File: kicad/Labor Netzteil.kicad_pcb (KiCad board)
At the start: 2 copper layers, 95.2 x 97.8 mm, 44 parts, among them J1 Out_1_01, J10 Sec 2 d, J11 Out_2_02, J12 Out_2_01, J13 OLED, J14 Fan, J15 Out_1, J16 NeoPixel, J17 Out_2, J2 Out_1_02, J3 Sec 1 d, J4 Sec 1 c, J5 Sec 1 b, J6 Sec 1 a, J7 Sec 2 a, J8 Sec 2 b, J9 Sec 2 c, U1 2-Relais-Modul, U2 LM7805_TO220, U3 L7812, U4 ESP-DevKitC, U5 74HC245, U6 DS18B20

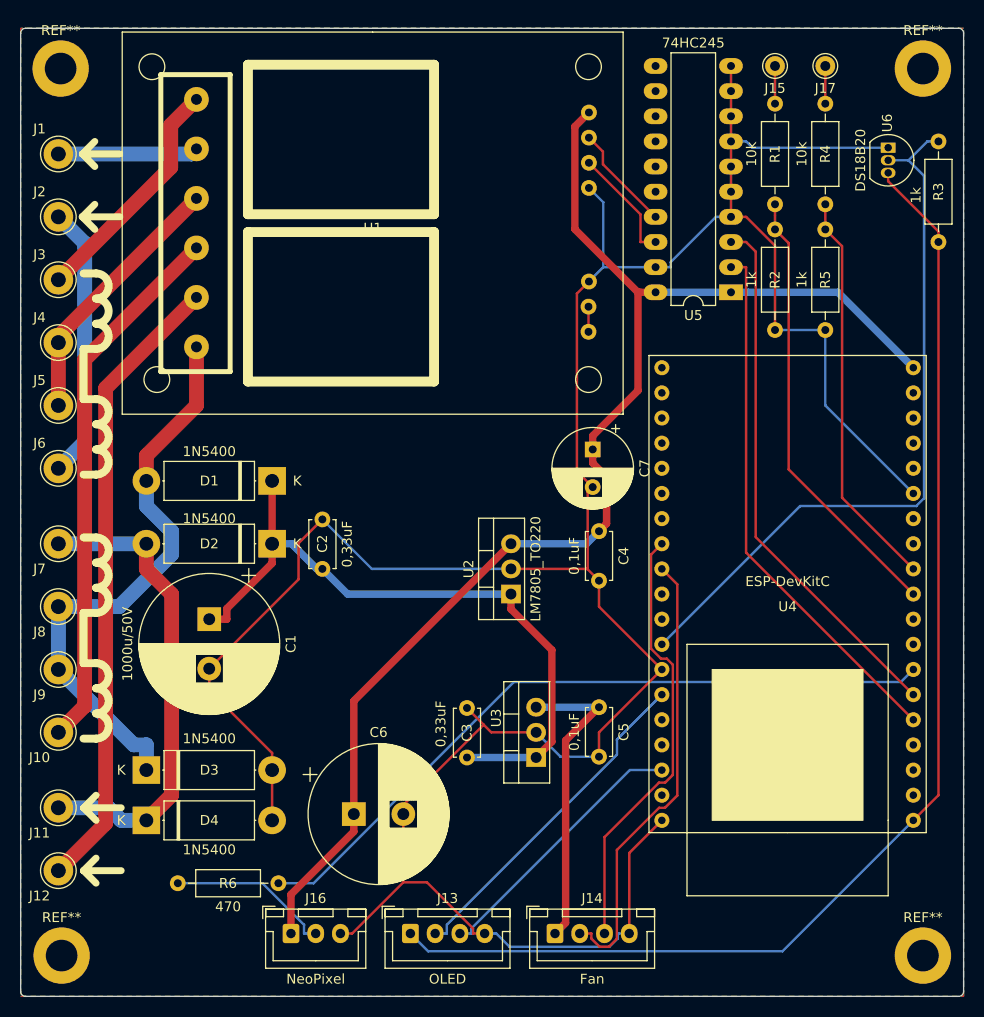
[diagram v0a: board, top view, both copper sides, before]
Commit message: Neueste Änderungen
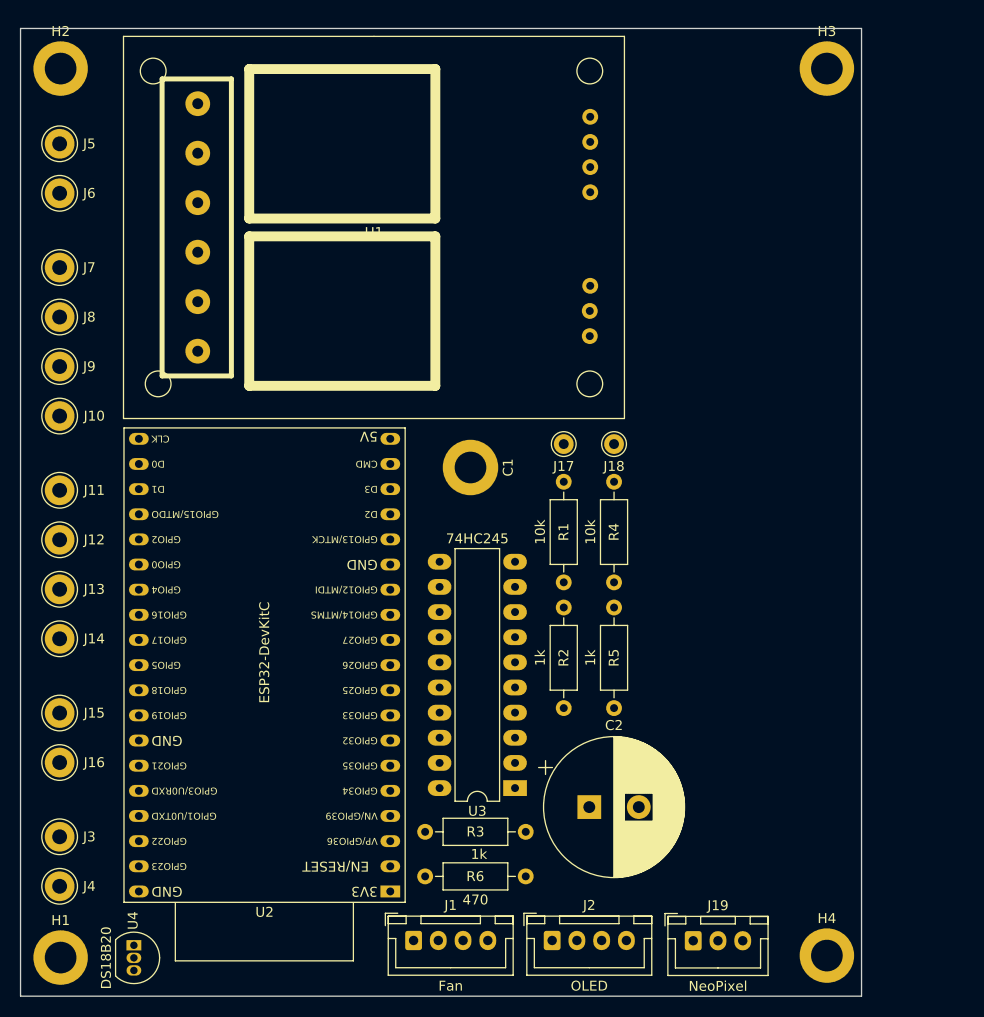
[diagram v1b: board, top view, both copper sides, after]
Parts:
- removed the C1 at (118.1, 96.5)
- removed C3: 0,33uF, Capacitor_THT:C_Disc_D4.7mm_W2.5mm_P5.00mm
- removed C4, C5: 0,1uF, Capacitor_THT:C_Disc_D4.7mm_W2.5mm_P5.00mm
- removed C6: 1000uF, Capacitor_THT:CP_Radial_D14.0mm_P5.00mm
- removed D1, D2, D3, D4: 1N5400, Diode_THT:D_5W_P12.70mm_Horizontal
- removed REF** (x4): MountingHole_3.2mm_M3_ISO7380_Pad, MountingHole:MountingHole_3.2mm_M3_ISO7380_Pad
- removed the U3 at (151.1, 110.5)
- removed the U4 at (176.5, 94.0)
- added H1: MountingHole_Pad, MountingHole:MountingHole_3.2mm_M3_ISO14580_Pad, F.Cu at (103.1, 130.7)
- added H2: MountingHole_Pad, MountingHole:MountingHole_3.2mm_M3_ISO14580_Pad, F.Cu at (103.1, 40.9)
- added H3: MountingHole_Pad, MountingHole:MountingHole_3.2mm_M3_ISO14580_Pad, F.Cu at (180.5, 40.9)
- added H4: MountingHole_Pad, MountingHole:MountingHole_3.2mm_M3_ISO14580_Pad, F.Cu at (180.5, 130.5)
- added J3: +5V In, Connector_Pin:Pin_D1.3mm_L11.0mm_LooseFit, F.Cu at (103.0, 118.5)
- added J4: GND 5V In, Connector_Pin:Pin_D1.3mm_L11.0mm_LooseFit, F.Cu at (103.0, 123.5)
- C1: renamed from C7; footprint Capacitor_THT:CP_Radial_D8.0mm_P3.80mm -> MountingHole:MountingHole_3.2mm_M3_DIN965_Pad
- C2: value 0,33uF -> 1000uF; footprint Capacitor_THT:C_Disc_D4.7mm_W2.5mm_P5.00mm -> Capacitor_THT:CP_Radial_D14.0mm_P5.00mm
- U2: value LM7805_TO220 -> ESP32-DevKitC; footprint Package_TO_SOT_THT:TO-220-3_Vertical -> PCM_Espressif:ESP32-DevKitC
- moved U4 110.9 mm to (110.5, 129.5)
- moved R3 72.7 mm to (150.1, 118.0), turned to 180 degrees
- moved U3 54.6 mm to (149.0, 113.6)
- moved R2 43.7 mm to (153.9, 95.3)
- moved R5 43.7 mm to (159.0, 95.3)
- moved J17 43.7 mm to (153.9, 78.8)
- moved J18 43.7 mm to (159.0, 78.8)
- moved R1 43.7 mm to (153.9, 82.6)
- moved R4 43.7 mm to (159.0, 82.6)
- moved J19 40.6 mm to (167.0, 129.0)
- moved C2 36.1 mm to (156.5, 115.5), turned to 0 degrees
- moved U2 32.4 mm to (136.4, 124.0), turned to 180 degrees
- moved R6 25.0 mm to (139.9, 122.5)
- moved J2 14.3 mm to (152.8, 129.0)
- moved J1 14.3 mm to (138.8, 129.0)
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- renumbered J14 to J1, J6 to J10, J7 to J11, J8 to J12, J9 to J13, J10 to J14, J11 to J15, J12 to J16, J15 to J17, J17 to J18, J16 to J19, J13 to J2, J1 to J5, J2 to J6, J3 to J7, J4 to J8, J5 to J9, U5 to U3, U6 to U4
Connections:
- C2 pad 1: Net-(C1-Pad1) -> 5V
- J1 pad 1: 12V -> 5V
- J2 pad 1: 3V3 -> 5V
- R3 pad 1: 3V3 -> 5V
- U1 pad 7: Net-(U1-Pad7) -> 5V
- U1 pad 8: Net-(U1-Pad7) -> 5V
- U2 pad 1: Net-(C1-Pad1) -> unconnected-(U2-3V3-Pad1)
- U2 pad 2: GND -> unconnected-(U2-CHIP_PU-Pad2)
- U2 pad 3: 5V -> unconnected-(U2-SENSOR_VP/GPIO36/ADC1_CH0-Pad3)
- U3 pad 11: Net-(U5-Pad11) -> unconnected-(U3-B7-Pad11)
- U3 pad 12: Net-(U5-Pad12) -> unconnected-(U3-B6-Pad12)
- U3 pad 13: Net-(U5-Pad13) -> unconnected-(U3-B5-Pad13)
- U3 pad 14: Net-(U5-Pad14) -> unconnected-(U3-B4-Pad14)
- U3 pad 15: Net-(U5-Pad15) -> unconnected-(U3-B3-Pad15)
- U3 pad 16: Net-(U5-Pad16) -> NeoPixel
- U3 pad 4: GND -> A2
- U4 pad 3: 3V3 -> 5V
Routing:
- net GND: track 301.1 -> 0.00 mm
- net 5V: track 137.3 -> 0.00 mm
- net 3V3: track 125.6 -> 0.00 mm
- net DS18B20: track 73.3 -> 0.00 mm
- net NeoPixel: track 73.1 -> 0.00 mm
- net Net-(C1-Pad1): track 69.7 -> 0.00 mm
- net Net-(J16-Pin_1): track 63.7 -> 0.00 mm
- net Net-(J12-Pin_1): track 58.7 -> 0.00 mm
- net Net-(J14-Pin_1): track 54.7 -> 0.00 mm
- net A1: track 54.2 -> 0.00 mm
- net A0: track 54.2 -> 0.00 mm
- net Net-(J11-Pin_1): track 48.4 -> 0.00 mm
- net TACHO: track 45.8 -> 0.00 mm
- net V_MON_1: track 45.2 -> 0.00 mm
- net PWM: track 44.3 -> 0.00 mm
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- removed copper zone on B.Cu, net GND
- removed copper zone on F.Cu, net GND
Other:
- board size 95.2 x 97.8 mm -> 85 x 97.8 mm

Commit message: Grundlegende Änderung der Schaltung, siehe README
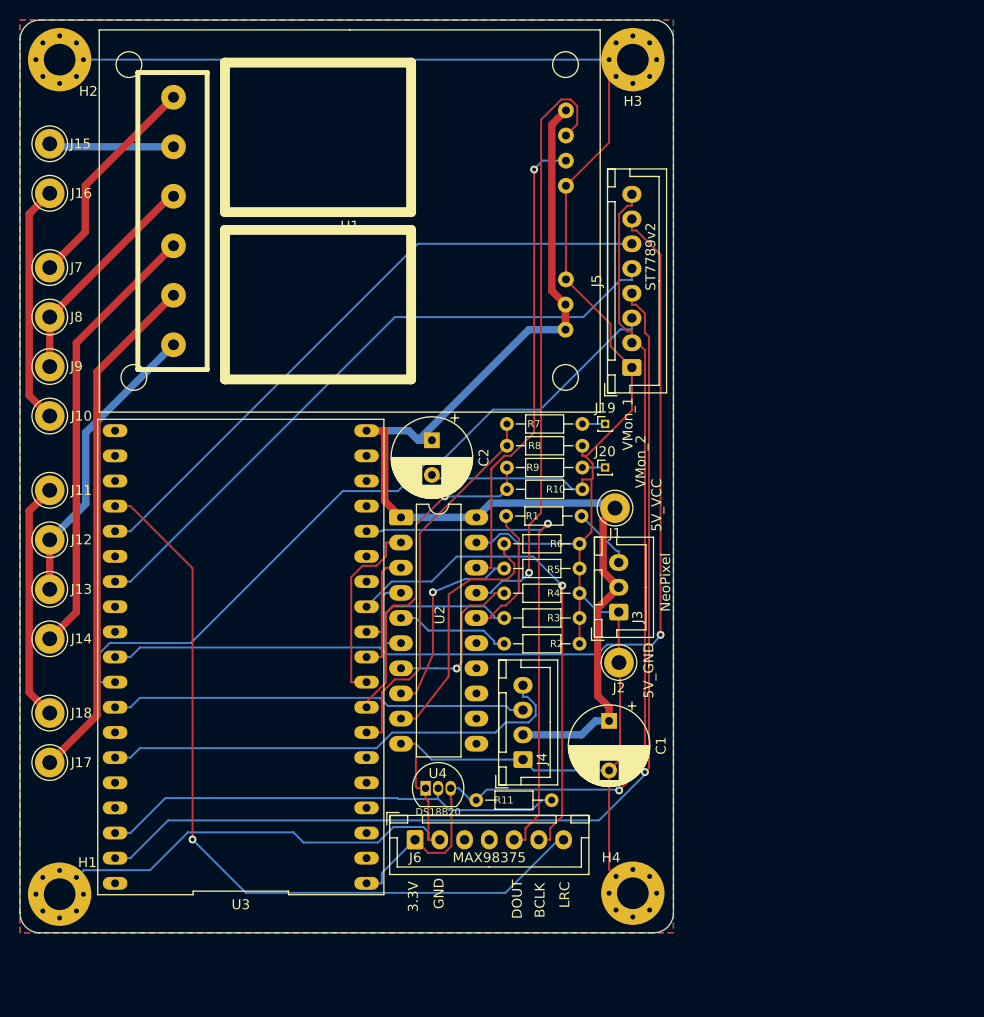
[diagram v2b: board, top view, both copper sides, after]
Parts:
- removed the J3 at (103.0, 118.5)
- added J5: ST7789v2, Connector_JST:JST_XH_B8B-XH-A_1x08_P2.50mm_Vertical, F.Cu at (160.8, 71.1)
- added J6: MAX98375, Connector_JST:JST_XH_B7B-XH-A_1x07_P2.50mm_Vertical, F.Cu at (138.9, 118.8)
- added R2: 10K, Resistor_THT:R_Axial_DIN0204_L3.6mm_D1.6mm_P7.62mm_Horizontal, F.Cu at (155.5, 99.0)
- added R3: 10K, Resistor_THT:R_Axial_DIN0204_L3.6mm_D1.6mm_P7.62mm_Horizontal, F.Cu at (155.5, 96.4)
- added R4: 10K, Resistor_THT:R_Axial_DIN0204_L3.6mm_D1.6mm_P7.62mm_Horizontal, F.Cu at (155.5, 93.9)
- added R5: 10K, Resistor_THT:R_Axial_DIN0204_L3.6mm_D1.6mm_P7.62mm_Horizontal, F.Cu at (155.5, 91.4)
- added R6: 10K, Resistor_THT:R_Axial_DIN0204_L3.6mm_D1.6mm_P7.62mm_Horizontal, F.Cu at (155.5, 88.9)
- C1: renamed from C2; footprint Capacitor_THT:CP_Radial_D14.0mm_P5.00mm -> Capacitor_THT:CP_Radial_D8.0mm_P5.00mm
- C2: renamed from C1; footprint MountingHole:MountingHole_3.2mm_M3_DIN965_Pad -> Capacitor_THT:CP_Radial_D8.0mm_P3.50mm
- H1: value MountingHole_Pad -> H1; footprint MountingHole:MountingHole_3.2mm_M3_ISO14580_Pad -> MountingHole:MountingHole_3.2mm_M3_Pad_Via
- H2: value MountingHole_Pad -> H2; footprint MountingHole:MountingHole_3.2mm_M3_ISO14580_Pad -> MountingHole:MountingHole_3.2mm_M3_Pad_Via
- H3: value MountingHole_Pad -> H3; footprint MountingHole:MountingHole_3.2mm_M3_ISO14580_Pad -> MountingHole:MountingHole_3.2mm_M3_Pad_Via
- H4: value MountingHole_Pad -> H4; footprint MountingHole:MountingHole_3.2mm_M3_ISO14580_Pad -> MountingHole:MountingHole_3.2mm_M3_Pad_Via
- J1: value Fan -> 5V_VCC; footprint Connector_JST:JST_XH_B4B-XH-A_1x04_P2.50mm_Vertical -> Connector_Pin:Pin_D1.3mm_L11.0mm_LooseFit
- J19: renamed from J17; value Out_1 -> VMon_1; footprint Connector_Pin:Pin_D1.0mm_L10.0mm -> Connector_PinHeader_1.00mm:PinHeader_1x01_P1.00mm_Vertical
- J2: value OLED -> 5V_GND; footprint Connector_JST:JST_XH_B4B-XH-A_1x04_P2.50mm_Vertical -> Connector_Pin:Pin_D1.3mm_L11.0mm_LooseFit
- J20: renamed from J18; value Out_2 -> VMon_2; footprint Connector_Pin:Pin_D1.0mm_L10.0mm -> Connector_PinHeader_1.00mm:PinHeader_1x01_P1.00mm_Vertical
- J4: value GND 5V In -> Fan; footprint Connector_Pin:Pin_D1.3mm_L11.0mm_LooseFit -> Connector_JST:JST_XH_B4B-XH-A_1x04_P2.50mm_Vertical
- R1: renamed from R6; footprint Resistor_THT:R_Axial_DIN0207_L6.3mm_D2.5mm_P10.16mm_Horizontal -> Resistor_THT:R_Axial_DIN0204_L3.6mm_D1.6mm_P7.62mm_Horizontal
- R10: renamed from R5; footprint Resistor_THT:R_Axial_DIN0207_L6.3mm_D2.5mm_P10.16mm_Horizontal -> Resistor_THT:R_Axial_DIN0204_L3.6mm_D1.6mm_P7.62mm_Horizontal
- R11: renamed from R3; value 1k -> 4.7K; footprint Resistor_THT:R_Axial_DIN0207_L6.3mm_D2.5mm_P10.16mm_Horizontal -> Resistor_THT:R_Axial_DIN0204_L3.6mm_D1.6mm_P7.62mm_Horizontal
- R7: renamed from R1; footprint Resistor_THT:R_Axial_DIN0207_L6.3mm_D2.5mm_P10.16mm_Horizontal -> Resistor_THT:R_Axial_DIN0204_L3.6mm_D1.6mm_P7.62mm_Horizontal
- R8: renamed from R2; footprint Resistor_THT:R_Axial_DIN0207_L6.3mm_D2.5mm_P10.16mm_Horizontal -> Resistor_THT:R_Axial_DIN0204_L3.6mm_D1.6mm_P7.62mm_Horizontal
- R9: renamed from R4; footprint Resistor_THT:R_Axial_DIN0207_L6.3mm_D2.5mm_P10.16mm_Horizontal -> Resistor_THT:R_Axial_DIN0204_L3.6mm_D1.6mm_P7.62mm_Horizontal
- U2: value ESP32-DevKitC -> 74HC245; footprint PCM_Espressif:ESP32-DevKitC -> Package_DIP:DIP-20_W7.62mm_LongPads
- U3: value 74HC245 -> ESP32-DEVKITC-32D; footprint Package_DIP:DIP-20_W7.62mm_LongPads -> RF_Module:ESP32-DevKitC-V4-b
- moved J4 48.5 mm to (149.8, 110.7), turned to 90 degrees
- moved J1 48.2 mm to (159.1, 85.3)
- moved R1 39.7 mm to (155.7, 86.1), turned to 180 degrees
- moved U2 37.8 mm to (137.5, 86.2), turned to 0 degrees
- moved J3 34.0 mm to (159.5, 95.8), turned to 90 degrees
- moved U4 33.5 mm to (140.0, 113.6), turned to 0 degrees
- moved U3 30.7 mm to (121.3, 100.3), turned to 90 degrees
- moved J2 28.9 mm to (159.5, 100.9)
- moved H4 20.6 mm to (160.9, 124.2)
- moved H3 19.6 mm to (160.9, 40.0)
- moved R8 17.3 mm to (148.2, 79.0), turned to 0 degrees
- moved R10 16.1 mm to (148.2, 83.4), turned to 0 degrees
- moved C1 8.93 mm to (158.5, 106.8), turned to -90 degrees
- moved H1 6.40 mm to (103.0, 124.3)
- moved R7 6.14 mm to (155.8, 76.8), turned to 180 degrees
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- renumbered J5 to J15, J6 to J16, J16 to J17, J15 to J18, J19 to J3
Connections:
- J2 pad 1: 5V -> GND
- J3 pad 1: 5V -> GND
- J3 pad 2: Net-(J19-Pin_2) -> 5V
- J3 pad 3: GND -> Net-(J3-Pin_3)
- R1 pad 1: Net-(J19-Pin_2) -> Net-(J3-Pin_3)
- R1 pad 2: NeoPixel -> NP_5V
- R11 pad 1: 5V -> 3.3V
- U2 pad 1: unconnected-(U2-3V3-Pad1) -> 5V
- U2 pad 10: V_MON_1 -> GND
- U2 pad 11: V_MON_2 -> unconnected-(U2-B7-Pad11)
- U2 pad 14: GND -> unconnected-(U2-B4-Pad14)
- U2 pad 16: unconnected-(U2-SD_DATA2/GPIO9-Pad16) -> NP_5V
- U2 pad 17: unconnected-(U2-SD_DATA3/GPIO10-Pad17) -> B1
- U2 pad 18: unconnected-(U2-CMD-Pad18) -> B0
- U2 pad 19: 5V -> GND
- U2 pad 2: unconnected-(U2-CHIP_PU-Pad2) -> A0
- U2 pad 20: unconnected-(U2-SD_CLK/GPIO6-Pad20) -> 5V
- U2 pad 3: unconnected-(U2-SENSOR_VP/GPIO36/ADC1_CH0-Pad3) -> A1
- U2 pad 4: unconnected-(U2-SENSOR_VN/GPIO39/ADC1_CH3-Pad4) -> NP_3.3V
- U2 pad 5: A0 -> Net-(U2-A3)
- U2 pad 6: A1 -> Net-(U2-A4)
- U2 pad 7: unconnected-(U2-32K_XP/GPIO32/ADC1_CH4-Pad7) -> Net-(U2-A5)
- U2 pad 8: unconnected-(U2-32K_XN/GPIO33/ADC1_CH5-Pad8) -> Net-(U2-A6)
- U2 pad 9: unconnected-(U2-DAC_1/ADC2_CH8/GPIO25-Pad9) -> Net-(U2-A7)
- U3 pad 1: 5V -> 3.3V
- U3 pad 10: GND -> A1
- U3 pad 11: unconnected-(U3-B7-Pad11) -> NP_3.3V
- U3 pad 12: unconnected-(U3-B6-Pad12) -> BLCK
- U3 pad 15: unconnected-(U3-B3-Pad15) -> DOUT
- U3 pad 16: NeoPixel -> unconnected-(U3-SD2-Pad16)
- U3 pad 17: B1 -> unconnected-(U3-SD3-Pad17)
- U3 pad 18: B0 -> unconnected-(U3-CMD-Pad18)
- U3 pad 19: GND -> 5V
- U3 pad 2: A0 -> unconnected-(U3-EN-Pad2)
- U3 pad 20: 5V -> unconnected-(U3-CLK-Pad20)
- U3 pad 3: A1 -> unconnected-(U3-SENSOR_VP-Pad3)
- U3 pad 4: A2 -> unconnected-(U3-SENSOR_VN-Pad4)
- U3 pad 5: GND -> unconnected-(U3-IO34-Pad5)
- U3 pad 6: GND -> unconnected-(U3-IO35-Pad6)
- U3 pad 7: GND -> V_MON_1
- U3 pad 8: GND -> V_MON_2
- U3 pad 9: GND -> A0
- U4 pad 3: 5V -> 3.3V
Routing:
- net GND: track 0.00 -> 328.3 mm
- net 5V: track 0.00 -> 116.8 mm
- net SDA: track 0.00 -> 106.8 mm, vias 0 -> 1
- net CS: track 0.00 -> 100.1 mm, vias 0 -> 1
- net 3.3V: track 0.00 -> 99.7 mm, vias 0 -> 1
- net LRCK/WS: track 0.00 -> 79.8 mm, vias 0 -> 1
- net SCL: track 0.00 -> 72.9 mm
- net RES: track 0.00 -> 66.0 mm
- net DC: track 0.00 -> 64.2 mm
- net B1: track 0.00 -> 60.7 mm, vias 0 -> 1
- net DOUT: track 0.00 -> 52.7 mm, vias 0 -> 1
- net Net-(J17-Pin_1): track 0.00 -> 52.4 mm
- net BLCK: track 0.00 -> 50.4 mm, vias 0 -> 1
- net TACHO: track 0.00 -> 48.1 mm
- net DS18B20: track 0.00 -> 47.6 mm
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- added copper zone on B.Cu, net GND
- added copper zone on F.Cu, net GND
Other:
- board size 85 x 97.8 mm -> 66 x 92.2 mm
- board text added: "3.3V"
- board text added: "BCLK"
- board text added: "DOUT"
- board text added: "GND"
- board text added: "LRC"
